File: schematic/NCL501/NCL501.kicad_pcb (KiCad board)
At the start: 2 copper layers, 137 x 107.5 mm, 37 parts, among them CN1 SCSI Intern, J1 SCSI extern, J2 Bus_ISA_8bit, U1 74LS175, U10 PAL16L8, U2 74LS125, U3 74LS14, U4 6116, U5 53C80, U6 27C128, U7 74LS688, U8 74LS688, U9 74LS245

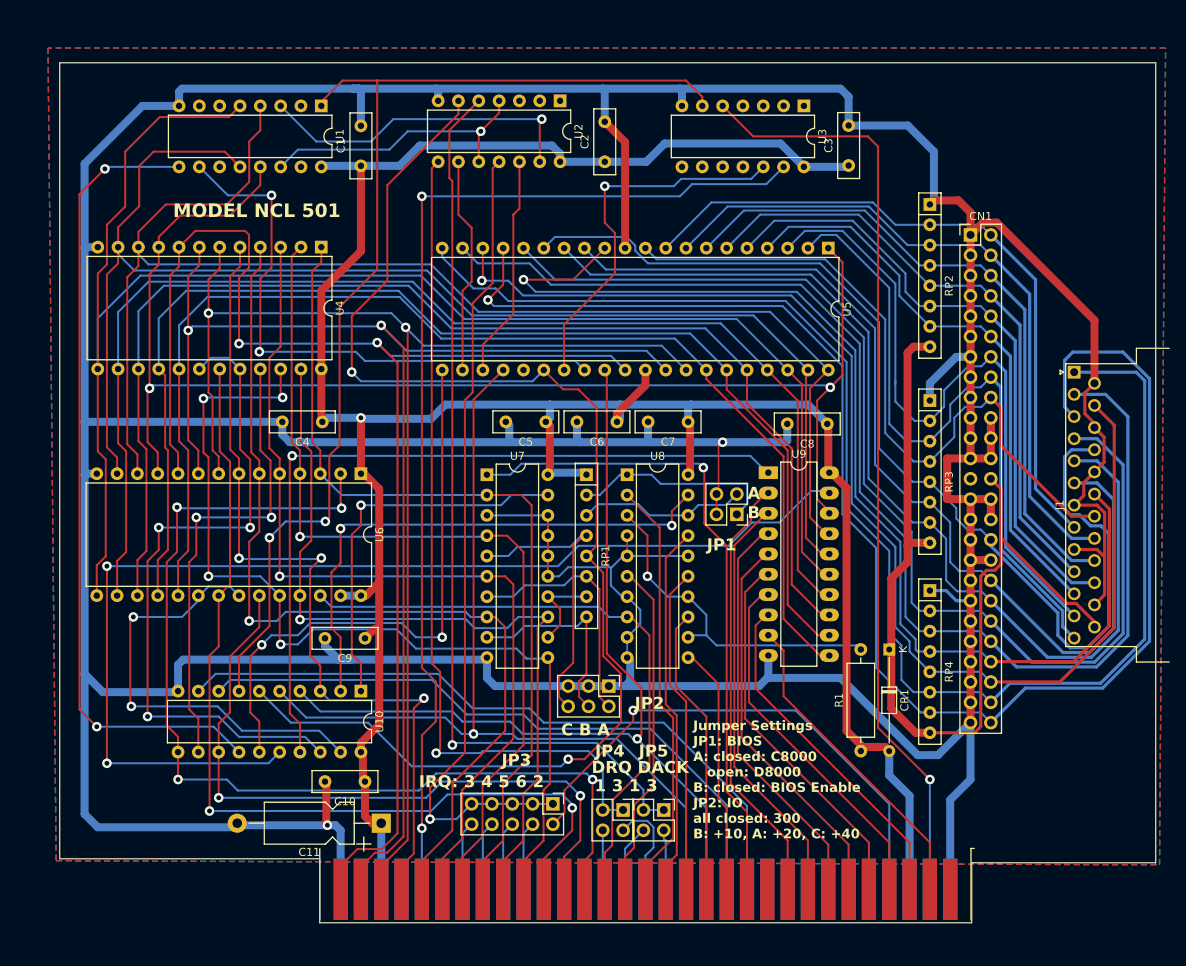
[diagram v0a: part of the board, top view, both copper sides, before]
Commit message: first manufactured Version
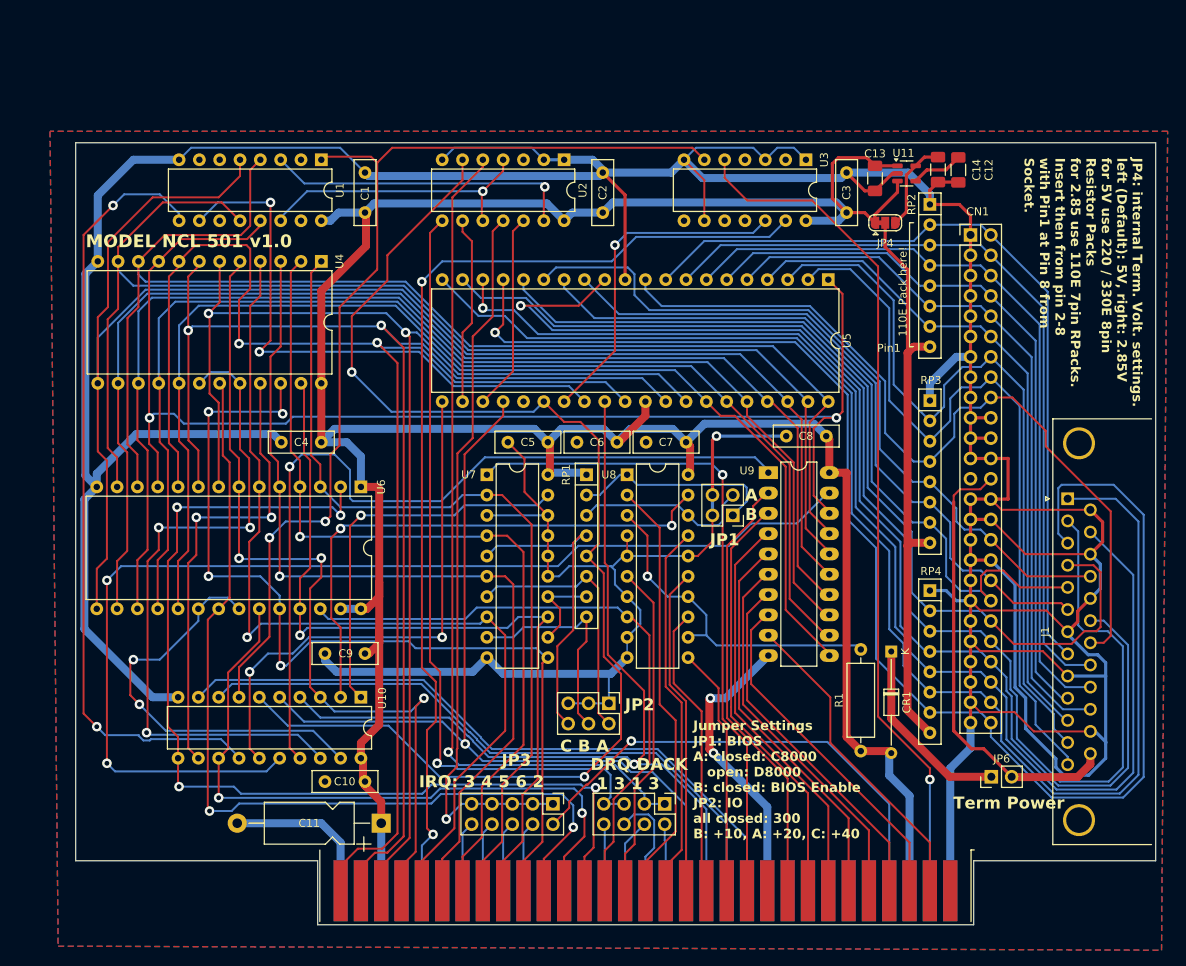
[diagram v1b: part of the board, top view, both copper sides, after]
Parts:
- removed JP5: DRQ, Connector_PinHeader_2.54mm:PinHeader_2x02_P2.54mm_Vertical
- added C12: 470p, Capacitor_SMD:C_1206_3216Metric_Pad1.33x1.80mm_HandSolder, F.Cu at (227.6, 56.9)
- added C13: 100n, Capacitor_SMD:C_1206_3216Metric_Pad1.33x1.80mm_HandSolder, F.Cu at (217.2, 58.0)
- added C14: 100n, Capacitor_SMD:C_1206_3216Metric_Pad1.33x1.80mm_HandSolder, F.Cu at (225.0, 56.9)
- added J4: DACK/DRQ, Connector_PinHeader_2.54mm:PinHeader_2x04_P2.54mm_Vertical, F.Cu at (190.9, 136.1)
- added JP6: TermPower, Connector_PinHeader_2.54mm:PinHeader_1x02_P2.54mm_Vertical, F.Cu at (231.7, 132.8)
- added U11: MIC5219-2.85YM5, Package_TO_SOT_SMD:SOT-23-5, F.Cu at (221.1, 57.3)
- J1: footprint Connector_Dsub:DSUB-25_Female_Horizontal_P2.77x2.54mm_EdgePinOffset9.40mm -> Connector_Dsub:DSUB-25_Female_Horizontal_P2.77x2.84mm_EdgePinOffset7.70mm_Housed_MountingHolesOffset9.12mm
- JP4: value DACK -> TRMPWRSEL; footprint Connector_PinHeader_2.54mm:PinHeader_2x02_P2.54mm_Vertical -> Jumper:SolderJumper-3_P1.3mm_Bridged12_RoundedPad1.0x1.5mm
- moved JP4 80.4 mm to (218.4, 63.5), turned to 0 degrees
- moved J1 15.8 mm to (241.2, 98.0)
- moved U2 7.38 mm to (178.3, 55.6)
- moved U3 6.74 mm to (208.5, 55.6)
- moved U1 6.73 mm to (148.0, 55.6)
- moved C2 6.36 mm to (183.1, 62.2)
- moved C3 5.89 mm to (213.6, 62.2)
- moved C1 5.86 mm to (153.4, 62.2)
- moved U5 3.94 mm to (211.3, 70.6)
- moved C5 2.55 mm to (176.3, 90.9)
- moved C7 2.55 mm to (193.5, 90.9)
- moved C4 2.54 mm to (148.0, 90.9)
- moved C6 2.54 mm to (184.9, 90.9)
- moved JP2 2.16 mm to (183.9, 123.6)
- moved C9 1.91 mm to (153.4, 117.3)
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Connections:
- net /W/~{R} renamed /~{RAMCE}
- CN1 pad 26: +5P -> Net-(CN1-Pin_26)
- CR1 pad 1: +5P -> Net-(CR1-K)
- J1 pad 25: +5P -> Net-(CN1-Pin_26)
- JP4 pad 1: Net-(JP4-Pin_1) -> +5V
- JP4 pad 2: /PDRQ3 -> +5P
- JP4 pad 3: Net-(JP4-Pin_1) -> Net-(JP4-B)
- U2 pad 1: unconnected-(U2-Pad1) -> GND
- U2 pad 2: unconnected-(U2-Pad2) -> GND
- U2 pad 8: Net-(JP4-Pin_1) -> Net-(J4-Pin_5)
- U3 pad 1: unconnected-(U3-Pad1) -> GND
- U3 pad 11: unconnected-(U3-Pad11) -> GND
- U3 pad 3: unconnected-(U3-Pad3) -> GND
- U3 pad 9: unconnected-(U3-Pad9) -> GND
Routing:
- net Net-(JP4-Pin_1): track 104.7 -> 0.00 mm, vias 1 -> 0
- net Net-(J4-Pin_5): track 0.00 -> 97.9 mm, vias 0 -> 1
- net Net-(CN1-Pin_26): track 0.00 -> 56.4 mm
- net /~{SATN}: track 135.0 -> 92.4 mm
- net +5P: track 114.4 -> 72.1 mm
- net /~{SBSY}: track 123.1 -> 86.1 mm
- net /~{SACK}: track 130.8 -> 96.0 mm
- net /~{SRST}: track 142.4 -> 115.8 mm
- net Net-(CR1-K): track 0.00 -> 23.9 mm
- net +5V: track 339.1 -> 359.9 mm, vias 1 -> 0
- net GND: track 777.4 -> 762.0 mm, vias 2 -> 3
- net /SD0: track 85.5 -> 100.4 mm
- net /SD3: track 77.7 -> 91.3 mm
- net /SDP: track 89.2 -> 102.6 mm
- net /SD2: track 83.5 -> 96.9 mm
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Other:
- board size 137 x 107.5 mm -> 135 x 97.8 mm
- board text added: "110E Pack here!"
- board text added: "JP4: internal Term. Volt. settings. left (Default): 5V, right: 2.85V for 5V use 220 / 330E 8pin Resistor Packs for 2.85 use 110E 7pin RPacks. Insert then from pin 2-8 with Pin1 at Pin 8 from Socket."
- board text added: "MODEL NCL 501 v1.0"
- board text added: "Pin1"
- board text added: "Term Power"
- board text removed: "MODEL NCL 501"
- board text removed: "TODO: Correctly place J1!"
